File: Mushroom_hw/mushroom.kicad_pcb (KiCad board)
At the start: 2 copper layers, 48 x 85 mm, 82 parts, among them Q1 2N7002, Q2 IRLML6401, Q3 ALS-PT19-315C, Q4 LED_RGB_WS2812B, Q5 LED_RGB_WS2812B, Q6 LED_RGB_WS2812B, SW1 SS-9, SW2 BUTTON, SW3 BUTTON, SW4 BUTTON

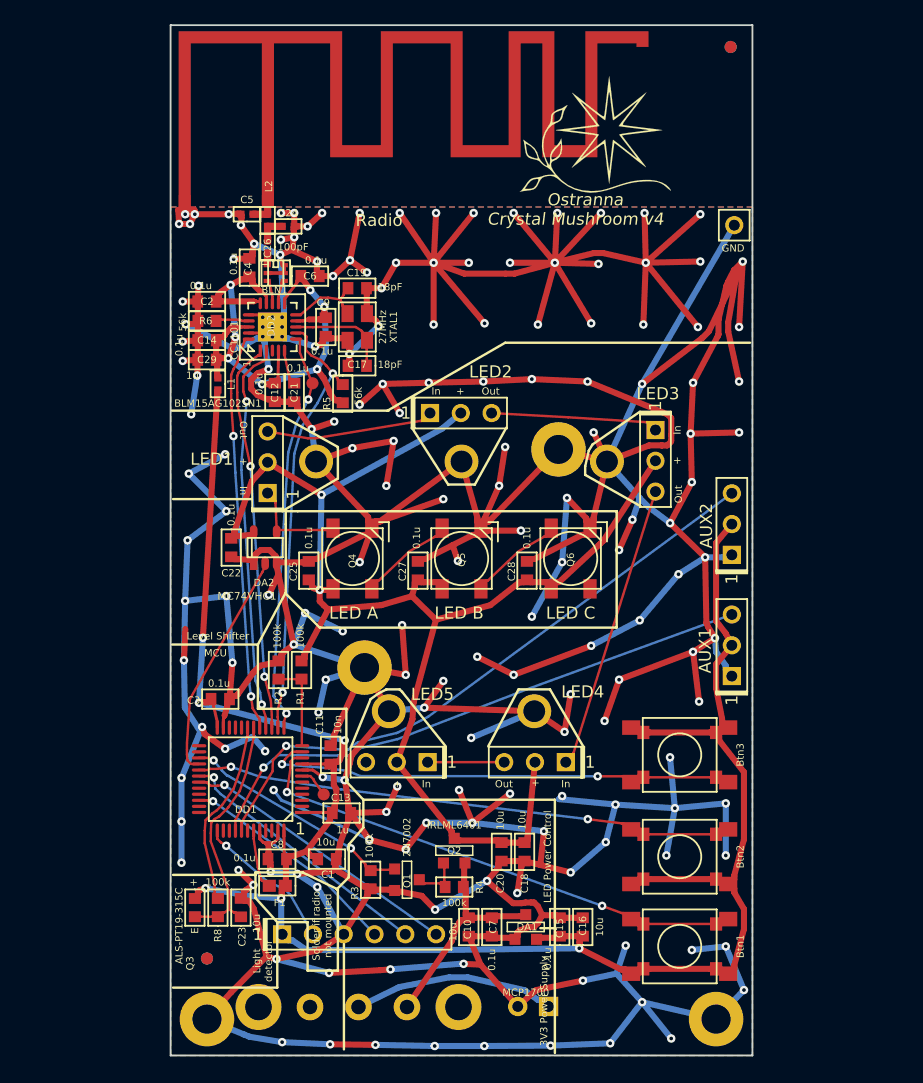
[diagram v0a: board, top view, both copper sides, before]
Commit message: + HW v5
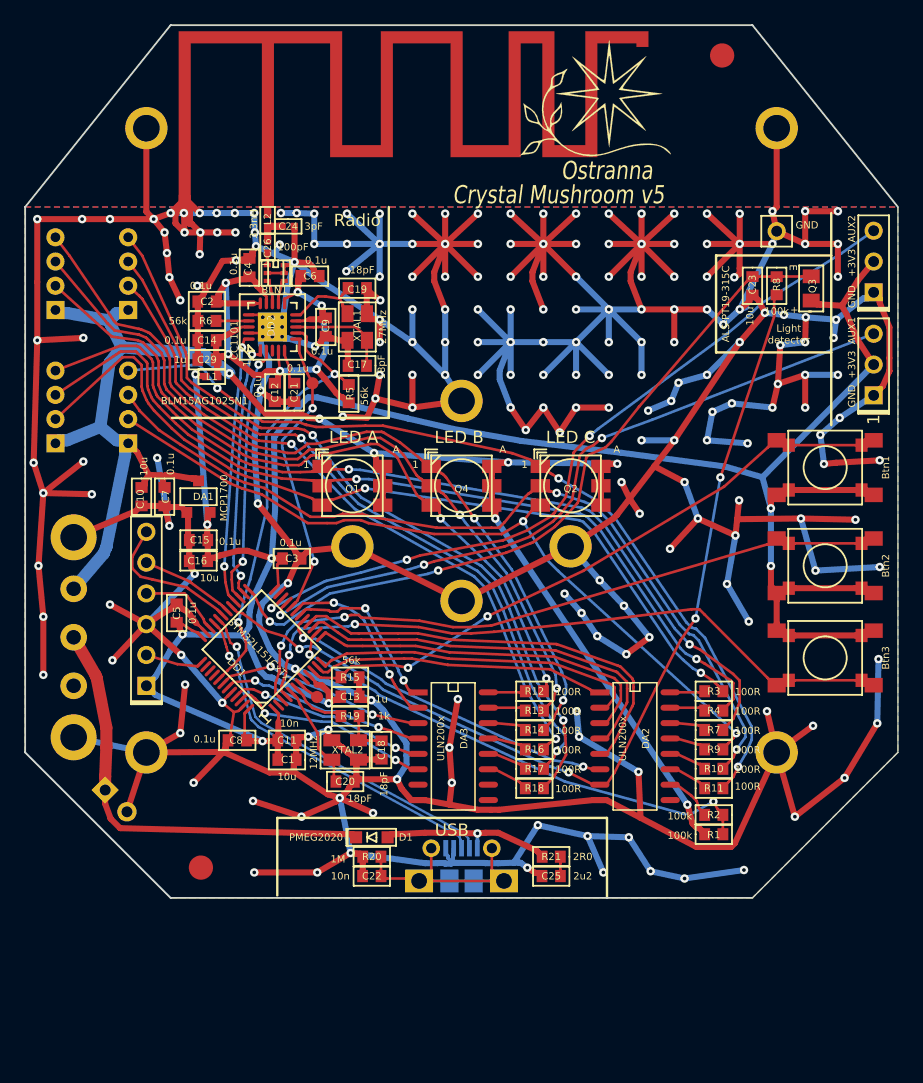
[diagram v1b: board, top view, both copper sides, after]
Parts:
- removed C27, C28: 0.1u, Capacitors:CAP_0603
- removed F1: Fuse0R, Resistors:RES_0603_FUSE
- removed Q5, Q6: LED_RGB_WS2812B, LEDs:LED_WS2812B
- removed RP3, RP4: REFPOINT, PCB:REF_POINT_1MM
- removed XL11, XL13, XL7, XL9: CONN_1, Connectors:SIL1_ROUND_1MM8
- removed XL12: CONN_3, Connectors:PLS-3
- added D1: PMEG2020, Diodes:SOD323, F.Cu at (220.6, 179.0)
- added DA3: ULN200x, SO_DIL_TSSOP:SO16_150MIL, F.Cu at (227.3, 170.8)
- added HOLE4: HOLE_METALLED, PCB:Hole2d2_out3d5mm, F.Cu at (228.0, 143.0)
- added HOLE6: HOLE_METALLED, PCB:Hole2d2_out3d5mm, F.Cu at (237.0, 155.0)
- added HOLE7: HOLE_METALLED, PCB:Hole2d2_out3d5mm, F.Cu at (219.0, 155.0)
- added HOLE8: HOLE_METALLED, PCB:Hole2d2_out3d5mm, F.Cu at (228.0, 159.5)
- added R10: 100R, Resistors:RES_0603, F.Cu at (248.8, 173.3)
- added R11: 100R, Resistors:RES_0603, F.Cu at (248.8, 174.9)
- added R12: 100R, Resistors:RES_0603, F.Cu at (234.0, 166.9)
- added R13: 100R, Resistors:RES_0603, F.Cu at (234.0, 168.5)
- added R14: 100R, Resistors:RES_0603, F.Cu at (234.0, 170.1)
- added R15: 56k, Resistors:RES_0603, F.Cu at (218.8, 165.8)
- added R16: 100R, Resistors:RES_0603, F.Cu at (234.0, 171.7)
- added R17: 100R, Resistors:RES_0603, F.Cu at (234.0, 173.3)
- added R18: 100R, Resistors:RES_0603, F.Cu at (234.0, 174.9)
- added R19: 1k, Resistors:RES_0603, F.Cu at (218.8, 169.0)
- added R20: 1M, Resistors:RES_0603, F.Cu at (220.6, 180.6)
- added R21: 2R0, Resistors:RES_0603, F.Cu at (235.4, 180.6)
- added R7: 100R, Resistors:RES_0603, F.Cu at (248.8, 170.1)
- added R9: 100R, Resistors:RES_0603, F.Cu at (248.8, 171.7)
- added XTAL2: 12MHz, Quartz:03225C4, F.Cu at (218.4, 171.8)
- ANT1: footprint Radio:ANT_IFA_MUSHROOM -> Antennas:ANT_IFA_MUSHROOM
- C18, C20: value 10u -> 18pF
- C22: value 0.1u -> 10n
- C24: value * -> 3pF
- C25: value 0.1u -> 2u2
- C5: value * -> 0.1u; footprint Capacitors:CAP_0402 -> Capacitors:CAP_0603
- DA1: footprint SOT:SOT23-3 -> SOT:SOT23-3A
- DA2: value MC74VHC1 -> ULN200x; footprint SOT:SOT23-5 -> SO_DIL_TSSOP:SO16_150MIL
- DD1: value STM32F030C8Tx -> STM32L151CxTx
- HOLE1, HOLE2, HOLE3, HOLE5: footprint PCB:Hole2d4_out4d5mm -> PCB:Hole2d2_out3d5mm
- L2: value * -> 3.3nH
- Q1: value 2N7002 -> LED_5050_new; footprint SOT:SOT23-3 -> LEDs:LED_5050
- Q2: value IRLML6401 -> LED_5050_new; footprint SOT:SOT23-3 -> LEDs:LED_5050
- Q3: footprint Resistors:RES_0603 -> Resistors:RES_0805
- Q4: value LED_RGB_WS2812B -> LED_5050_new; footprint LEDs:LED_WS2812B -> LEDs:LED_5050
- R3, R4: value 100k -> 100R
- RP1, RP2: footprint PCB:REF_POINT_1MM -> PCB:REF_POINT_2MM
- XL10, XL4, XL6, XL8: value CONN_3 -> CONN_4; footprint Connectors:PLS-3 -> Connectors:WB-04(MW-4M); moved to B.Cu
- XL5: value CONN_1 -> USB_MICRO_2H; footprint Connectors:SIL1_ROUND_1MM8 -> Connectors:USBmicro_MOLEX_1050170001; moved to B.Cu
- moved HOLE3 87.2 mm to (254.0, 120.5)
- moved Q3 72.1 mm to (256.8, 133.7), turned to 90 degrees
- moved R8 69.0 mm to (254.0, 133.5), turned to 270 degrees
- moved C23 66.4 mm to (252.0, 133.5), turned to 270 degrees
- moved XL10 54.1 mm to (200.5, 132.5), turned to 90 degrees
- moved XL8 51.2 mm to (194.5, 132.5), turned to 90 degrees
- moved C10 44.6 mm to (201.6, 150.9)
- moved C7 44.6 mm to (203.5, 150.9)
- moved DA1 44.6 mm to (206.3, 150.9)
- moved C16 43.8 mm to (206.3, 156.2), turned to 180 degrees
- moved C15 43.7 mm to (206.3, 154.5), turned to 180 degrees
- moved HOLE1 43.1 mm to (202.0, 120.5)
- moved SW2 41.3 mm to (258.0, 148.5)
- moved SW1 38.5 mm to (196.0, 162.5), turned to 270 degrees
- moved XL3 38.4 mm to (199.5, 176.0), turned to 315 degrees
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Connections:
- C18 pad 1: GND -> Net-(C18-Pad1)
- C18 pad 2: PwrUnst -> GND
- C20 pad 1: GND -> Net-(C20-Pad1)
- C20 pad 2: PwrUnst -> GND
- C22 pad 1: PwrUnst -> Net-(C22-Pad1)
- C25 pad 1: PwrUnst -> GND
- C25 pad 2: GND -> Net-(C25-Pad2)
- C5 pad 1: /ANT2 -> +3.3V
- DA2 pad 1: GND -> /R1
- DA2 pad 2: /WS_CTRL -> /G1
- DA2 pad 3: GND -> /B1
- DA2 pad 4: /DIN0 -> /R2
- DA2 pad 5: PwrUnst -> /G2
- DD1 pad 11: /BTN3 -> /R1
- DD1 pad 12: /ADC_BATTERY -> /G1
- DD1 pad 13: /CC_GDO0 -> /B1
- DD1 pad 14: /CC_CS -> /ADC_BATTERY
- DD1 pad 15: /CC_SCK -> /R2
- DD1 pad 16: /CC_MISO -> /G2
- DD1 pad 17: /CC_MOSI -> /B2
- DD1 pad 18: /ADC_LUM -> /R3
- DD1 pad 19: /MEAS_LUM -> /G3
- DD1 pad 2: Net-(DD1-Pad2) -> (no net)
- DD1 pad 20: Net-(DD1-Pad20) -> /CC_GDO0
- DD1 pad 21: Net-(DD1-Pad21) -> /AUX1
- DD1 pad 22: Net-(DD1-Pad22) -> /AUX2
- DD1 pad 25: Net-(DD1-Pad25) -> /ADC_LUM
- DD1 pad 26: Net-(DD1-Pad26) -> /CC_SCK
- DD1 pad 27: /PWR_EN -> /CC_MISO
- DD1 pad 28: /WS_CTRL -> /CC_MOSI
- DD1 pad 29: /BTN2 -> /MEASURE_EN
- DD1 pad 3: Net-(DD1-Pad3) -> /BTN2
- DD1 pad 32: Net-(DD1-Pad32) -> /D-
- DD1 pad 33: Net-(DD1-Pad33) -> /D+
- DD1 pad 35: Net-(DD1-Pad35) -> GND
- DD1 pad 36: Net-(DD1-Pad36) -> +3.3V
- DD1 pad 38: Net-(DD1-Pad38) -> (no net)
- DD1 pad 39: Net-(DD1-Pad39) -> (no net)
- DD1 pad 4: Net-(DD1-Pad4) -> /BTN3
- DD1 pad 40: /AUX1 -> (no net)
- DD1 pad 41: /AUX2 -> /CC_CS
- DD1 pad 42: Net-(DD1-Pad42) -> /B3
- DD1 pad 43: /NO_RADIO -> /R4
- DD1 pad 45: Net-(DD1-Pad45) -> /G4
- DD1 pad 46: Net-(DD1-Pad46) -> /B4
- DD1 pad 5: Net-(DD1-Pad5) -> Net-(C20-Pad1)
- DD2 pad 3: Net-(DD2-Pad3) -> (no net)
- Q1 pad 1: /PWR_EN -> /BO1
- Q1 pad 2: GND -> /GO1
- Q1 pad 3: Net-(Q1-Pad3) -> /RO1
- Q2 pad 1: Net-(Q1-Pad3) -> /BO2
- Q2 pad 2: +BATT -> /GO2
- Q2 pad 3: PwrUnst -> /RO2
- Q4 pad 1: PwrUnst -> /BO3
- Q4 pad 2: Net-(Q4-Pad2) -> /GO3
- Q4 pad 3: GND -> /RO3
- Q4 pad 4: /DIN0 -> +BATT
- R1 pad 1: PwrUnst -> +BATT
- R2 pad 2: GND -> Net-(DA2-Pad10)
- R3 pad 1: /PWR_EN -> Net-(DA2-Pad16)
- R3 pad 2: GND -> /RO1
- R4 pad 1: +BATT -> Net-(DA2-Pad15)
- R4 pad 2: Net-(Q1-Pad3) -> /GO1
- R8 pad 2: /MEAS_LUM -> /MEASURE_EN
- SW1 pad 3: Net-(SW1-Pad3) -> (no net)
- SW1 pad H: (no net) -> GND
- XL10 pad 1: /DIN3 -> +BATT
- XL10 pad 2: PwrUnst -> /RO4
- XL10 pad 3: /DIN4 -> /GO4
- XL4 pad 1: /DIN0 -> +BATT
- XL4 pad 2: PwrUnst -> /RO1
- XL4 pad 3: /DIN1 -> /GO1
- XL5 pad 1: GND -> Net-(D1-PadA)
- XL6 pad 1: /DIN1 -> +BATT
- XL6 pad 2: PwrUnst -> /RO2
- XL6 pad 3: /DIN2 -> /GO2
- XL8 pad 1: /DIN2 -> +BATT
- XL8 pad 2: PwrUnst -> /RO3
- XL8 pad 3: /DIN3 -> /GO3
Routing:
- net +BATT: track 18.7 -> 135.9 mm, vias 0 -> 7
- net PwrUnst: track 116.2 -> 0.00 mm, vias 2 -> 0
- net /MEASURE_EN: track 0.00 -> 78.1 mm, vias 0 -> 4
- net /BO1: track 0.00 -> 73.5 mm, vias 0 -> 2
- net /GO1: track 0.00 -> 71.8 mm, vias 0 -> 2
- net /BO2: track 0.00 -> 70.5 mm, vias 0 -> 3
- net /GO2: track 0.00 -> 70.1 mm, vias 0 -> 2
- net /RO1: track 0.00 -> 69.9 mm, vias 0 -> 2
- net /BO3: track 0.00 -> 66.7 mm, vias 0 -> 2
- net /RO2: track 0.00 -> 64.0 mm, vias 0 -> 2
- net /BO4: track 0.00 -> 63.3 mm, vias 0 -> 2
- net /GO3: track 0.00 -> 63.0 mm, vias 0 -> 2
- net /GO4: track 0.00 -> 59.8 mm, vias 0 -> 2
- net /RO3: track 0.00 -> 59.3 mm, vias 0 -> 2
- net /RO4: track 0.00 -> 55.6 mm, vias 0 -> 2
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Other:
- board size 48 x 85 mm -> 72 x 72 mm
- net class Default: trace_width 0.25 -> 0.22
- board text added: "+3V3"
- board text added: "+3v3"
- board text added: "Crystal Mushroom v5"
- board text added: "ON"
- board text added: "USB"
- board text removed: "3V3 Power Supply"
- board text removed: "Crystal Mushroom v4"
- board text removed: "In"
- board text removed: "LED Power Control"
- board text removed: "LED5"
- board text removed: "Level Shifter"
- board text removed: "MCU"
- board text removed: "Out"
- board text removed: "Solder if radio not mounted"
